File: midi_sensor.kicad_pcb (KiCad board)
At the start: 2 copper layers, 20 x 77 mm, 45 parts, among them J1 Conn_01x14, Q1 BCX54, U1 CJ431, U2 LM393, U3 QRE1113, U4 LM321, U5 CJ431

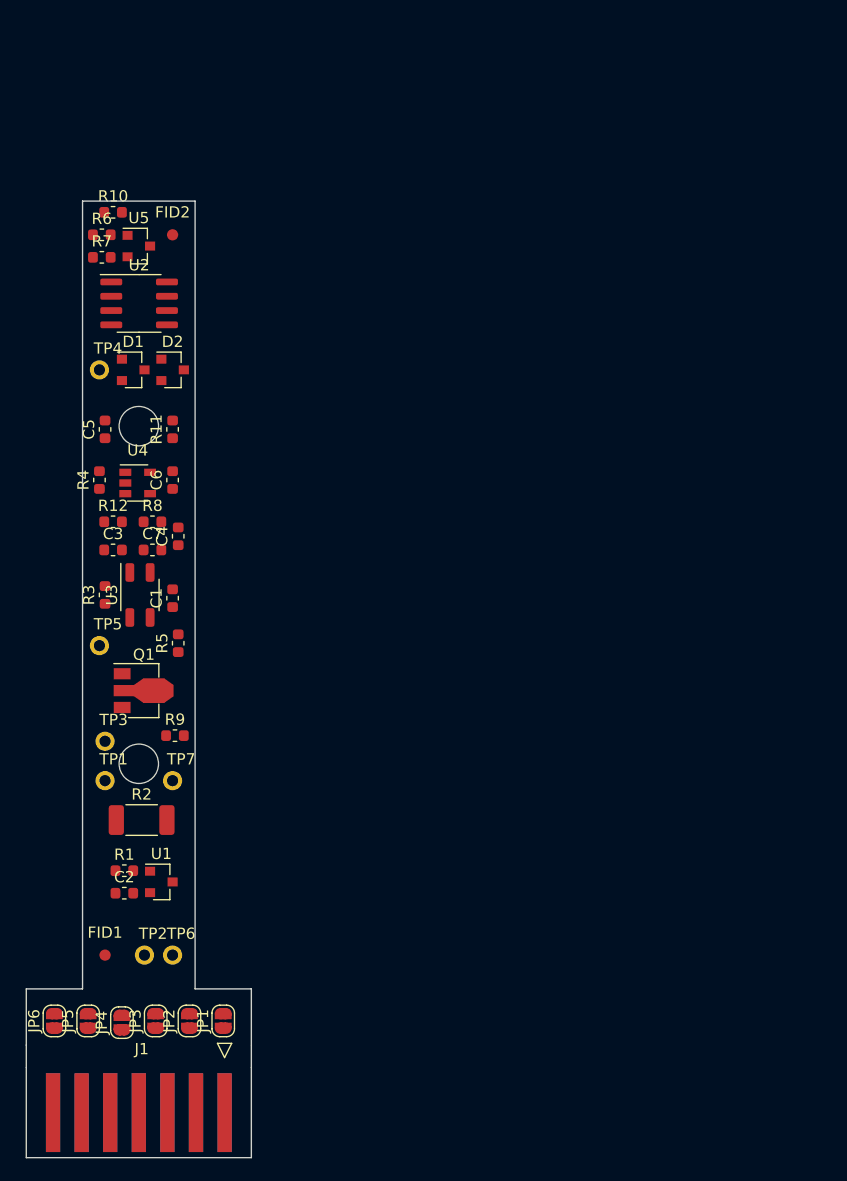
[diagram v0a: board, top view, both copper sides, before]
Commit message: Add files via upload
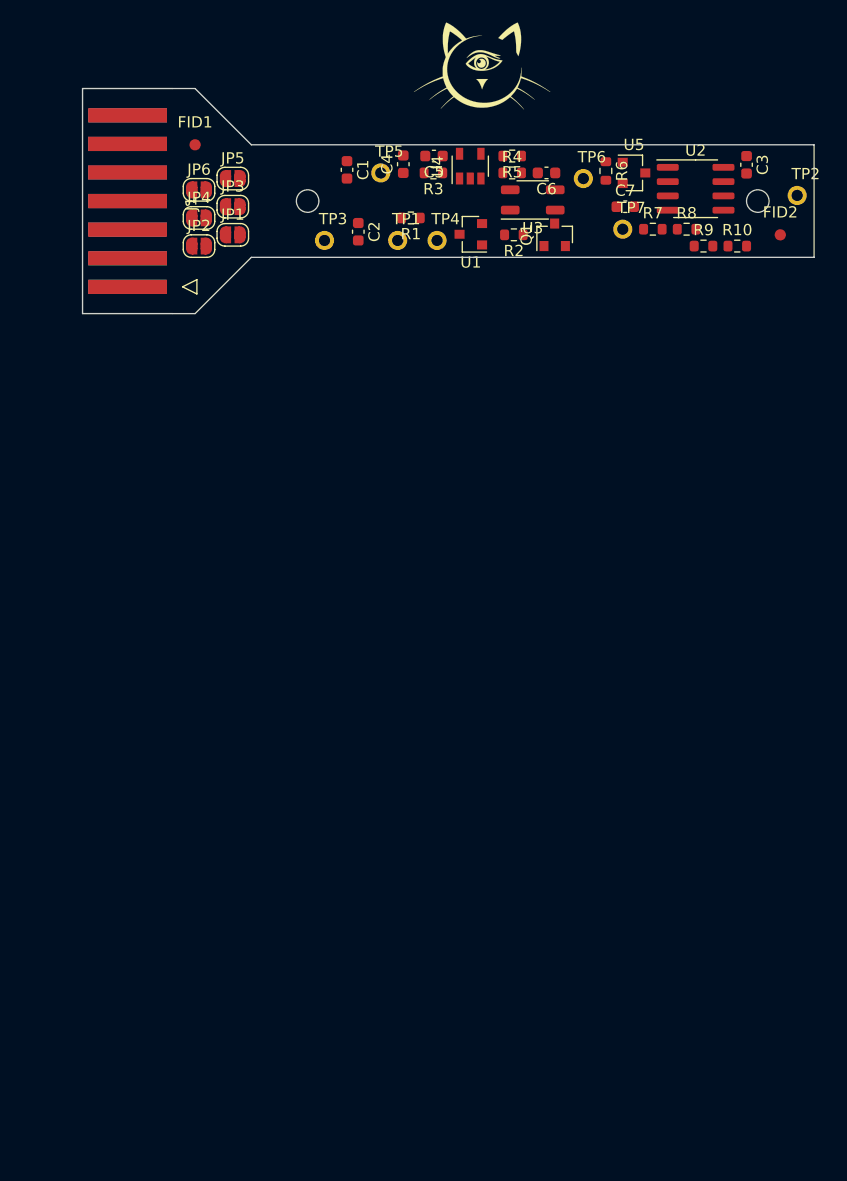
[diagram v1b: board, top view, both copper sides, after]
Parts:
- removed D1, D2: BAT54C, Package_TO_SOT_SMD:SOT-23
- removed R11: 1.1 1%, Resistor_SMD:R_0603_1608Metric
- removed R12: 13k, Resistor_SMD:R_0603_1608Metric
- added G1: LOGO, midi_sensor:stamp, F.Cu at (35.5, -12.0)
- H1, H2: footprint midi_sensor:hole_D3.5mm -> midi_sensor:hole_D2mm
- Q1: value BCX54 -> BC847; footprint Package_TO_SOT_SMD:SOT-89-3 -> Package_TO_SOT_SMD:SOT-23
- R10: value 3.3k 1% -> 13k 1%
- R2: value 4.7 1% 2010 -> 51 1%; footprint Resistor_SMD:R_2010_5025Metric -> Resistor_SMD:R_0603_1608Metric
- R4: value 1.1k -> 1k
- R7: value 1.1k 1% -> 30k 1%
- R8: value 1.1 1% -> 30k 1%
- R9: value 13k -> 30k 1%
- moved TP2 89.0 mm to (63.5, -0.50)
- moved J1 85.1 mm to (0.00, 0.00), turned to 270 degrees
- moved TP6 78.1 mm to (44.5, -2.00)
- moved JP5 75.9 mm to (13.3, -2.00), turned to 0 degrees
- moved JP6 75.0 mm to (10.3, -1.00), turned to 0 degrees
- moved JP3 72.7 mm to (13.3, 0.50), turned to 0 degrees
- moved FID1 72.4 mm to (10.0, -5.00)
- moved JP4 71.8 mm to (10.3, 1.50), turned to 0 degrees
- moved JP1 69.9 mm to (13.3, 3.00), turned to 0 degrees
- moved JP2 68.9 mm to (10.3, 4.00), turned to 0 degrees
- moved C3 65.9 mm to (59.0, -3.23), turned to 270 degrees
- moved R9 64.0 mm to (55.2, 4.00)
- moved U1 63.8 mm to (34.5, 2.95), turned to 180 degrees
- moved R1 63.3 mm to (29.2, 1.50), turned to 180 degrees
- moved TP7 63.3 mm to (48.0, 2.50)
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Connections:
- R10 pad 1: Net-(C7-Pad1) -> Net-(R10-Pad1)
- R10 pad 2: Net-(R10-Pad2) -> GND
- R2 pad 1: Net-(Q1-Pad3) -> Net-(Q1-Pad2)
- R9 pad 1: Net-(R7-Pad2) -> Net-(C7-Pad1)
- R9 pad 2: Net-(D1-Pad1) -> Net-(R10-Pad1)
- TP4 pad 1: Net-(Q1-Pad3) -> Net-(Q1-Pad2)
- U1 pad 1: Net-(Q1-Pad3) -> Net-(Q1-Pad2)
- U2 pad 1: Net-(D1-Pad3) -> /COMP_OUT_HI
- U2 pad 5: Net-(R10-Pad2) -> Net-(R10-Pad1)
- U2 pad 7: Net-(D2-Pad3) -> /COMP_OUT_LO
- U3 pad 2: Net-(Q1-Pad2) -> Net-(Q1-Pad3)
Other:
- board size 20 x 77 mm -> 57 x 20 mm
- rule pad_to_mask_clearance: 0.051 -> 0

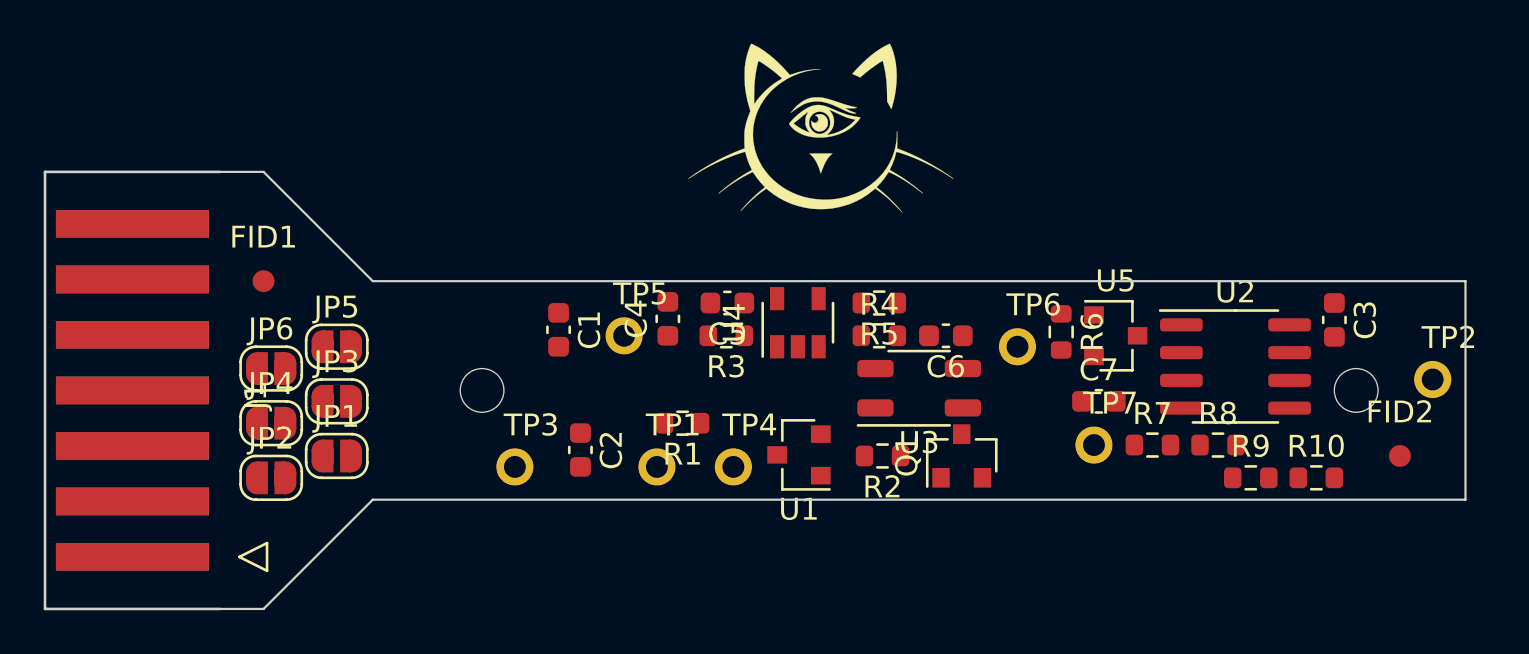
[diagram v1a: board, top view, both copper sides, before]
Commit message: Add files via upload
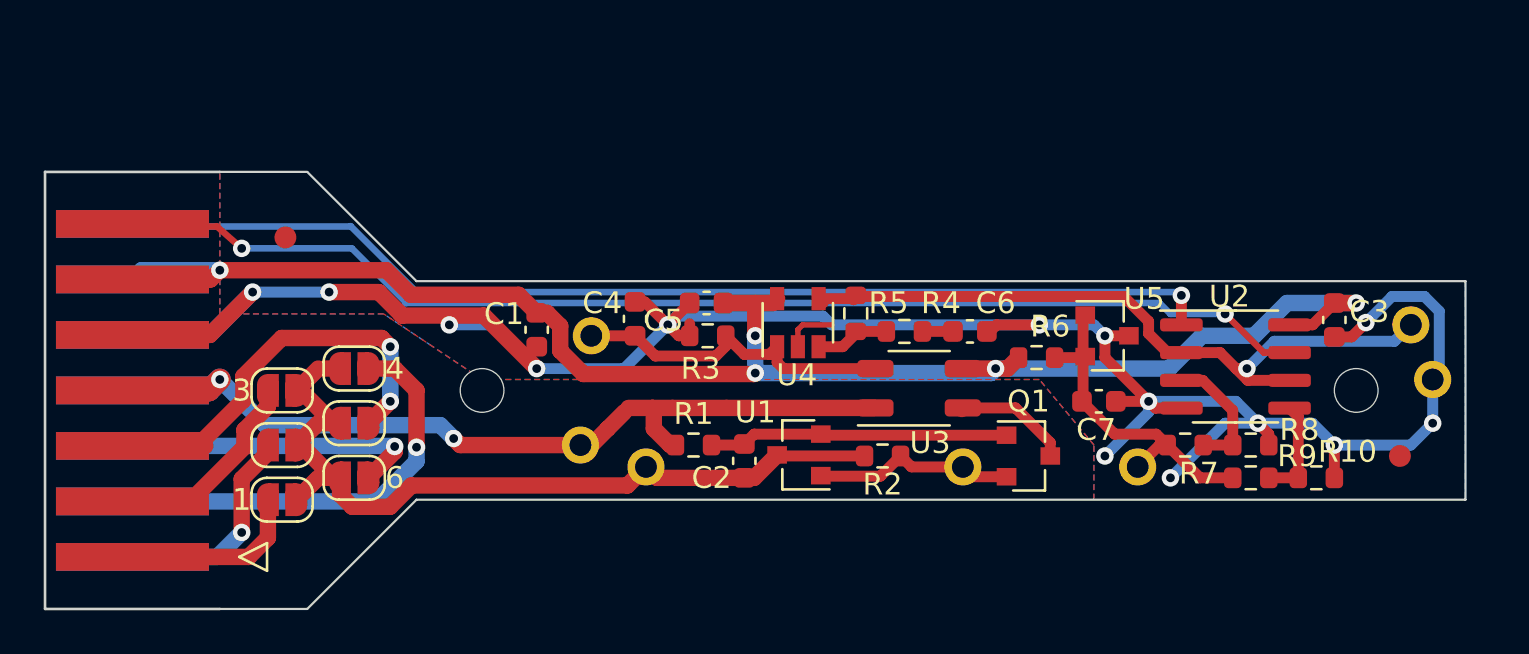
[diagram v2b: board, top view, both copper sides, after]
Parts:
- G1: moved to B.Cu
- moved TP6 18.0 mm to (62.5, -3.00)
- moved G1 12.0 mm to (34.5, 0.00), turned to 180 degrees
- moved TP4 10.5 mm to (42.0, 3.50)
- moved C2 7.52 mm to (32.0, 3.23)
- moved JP6 6.28 mm to (14.2, 4.00), turned to 180 degrees
- moved JP4 4.55 mm to (14.2, -1.00), turned to 180 degrees
- moved JP5 3.59 mm to (14.2, 1.50), turned to 180 degrees
- moved JP1 3.20 mm to (10.8, 5.00)
- moved TP3 3.16 mm to (24.5, 2.50)
- moved Q1 3.05 mm to (45.0, 3.00), turned to 0 degrees
- moved JP3 2.55 mm to (10.8, 0.00)
- moved FID1 2.24 mm to (11.0, -7.00)
- moved TP7 2.24 mm to (50.0, 3.50)
- moved R6 1.63 mm to (45.4, -1.50), turned to 0 degrees
- moved JP2 1.58 mm to (10.8, 2.50)
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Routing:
- net GND: track 0.00 -> 113.3 mm, vias 0 -> 14
- net +5V: track 0.00 -> 76.3 mm, vias 0 -> 5
- net /COMP_OUT_LO: track 0.00 -> 55.4 mm, vias 0 -> 2
- net /COMP_OUT_HI: track 0.00 -> 49.7 mm, vias 0 -> 1
- net /+VCC_PULSE: track 0.00 -> 42.4 mm, vias 0 -> 2
- net /GND_PULSE: track 0.00 -> 37.4 mm
- net Net-(R5-Pad1): track 0.00 -> 32.9 mm, vias 0 -> 1
- net Net-(J1-Pad5): track 0.00 -> 23.9 mm, vias 0 -> 2
- net Net-(J1-Pad4): track 0.00 -> 19.6 mm, vias 0 -> 1
- net Net-(C7-Pad1): track 0.00 -> 15.6 mm
- net Net-(C4-Pad1): track 0.00 -> 15.4 mm
- net Net-(J1-Pad3): track 0.00 -> 15.1 mm
- net Net-(J1-Pad6): track 0.00 -> 13.9 mm, vias 0 -> 1
- net Net-(C2-Pad1): track 0.00 -> 13.7 mm
- net Net-(J1-Pad2): track 0.00 -> 9.96 mm, vias 0 -> 1
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- added copper zone on B.Cu, net GND
- added copper zone on F.Cu, net GND
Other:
- outline, holes or cut-outs redrawn
- board text added: "1"
- board text added: "3"
- board text added: "4"
- board text added: "6"
- board text added: "midi_sensor 1.2"
